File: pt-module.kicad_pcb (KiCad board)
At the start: 2 copper layers, 107 parts, among them J1 M12 in, J10 M12, J2 Ethercon out, J3 PWR in, J4 M12 out, J5 Ethercon out, J6 M12, J7 M12, J8 USB_OTG, J9 M12, SW1 pwr-source switch, SW10 SW_Push, SW11 SW_Push, SW12 SW_Push, SW13 SW_Push, SW2 SW_Push, SW3 SW_Push, SW4 SW_Push, SW5 SW_Push, SW6 SW_Push, SW7 SW_Push, SW8 SW_Push, SW9 SW_Push, U1 MCP16331, U10 LH1526, U2 MCP16331, U3 SN65HVD72, U4 SN65HVD72, U5 DG411, U6 LH1526, U7 FT230XS, U8 STM32F334R8Tx, U9 DG411

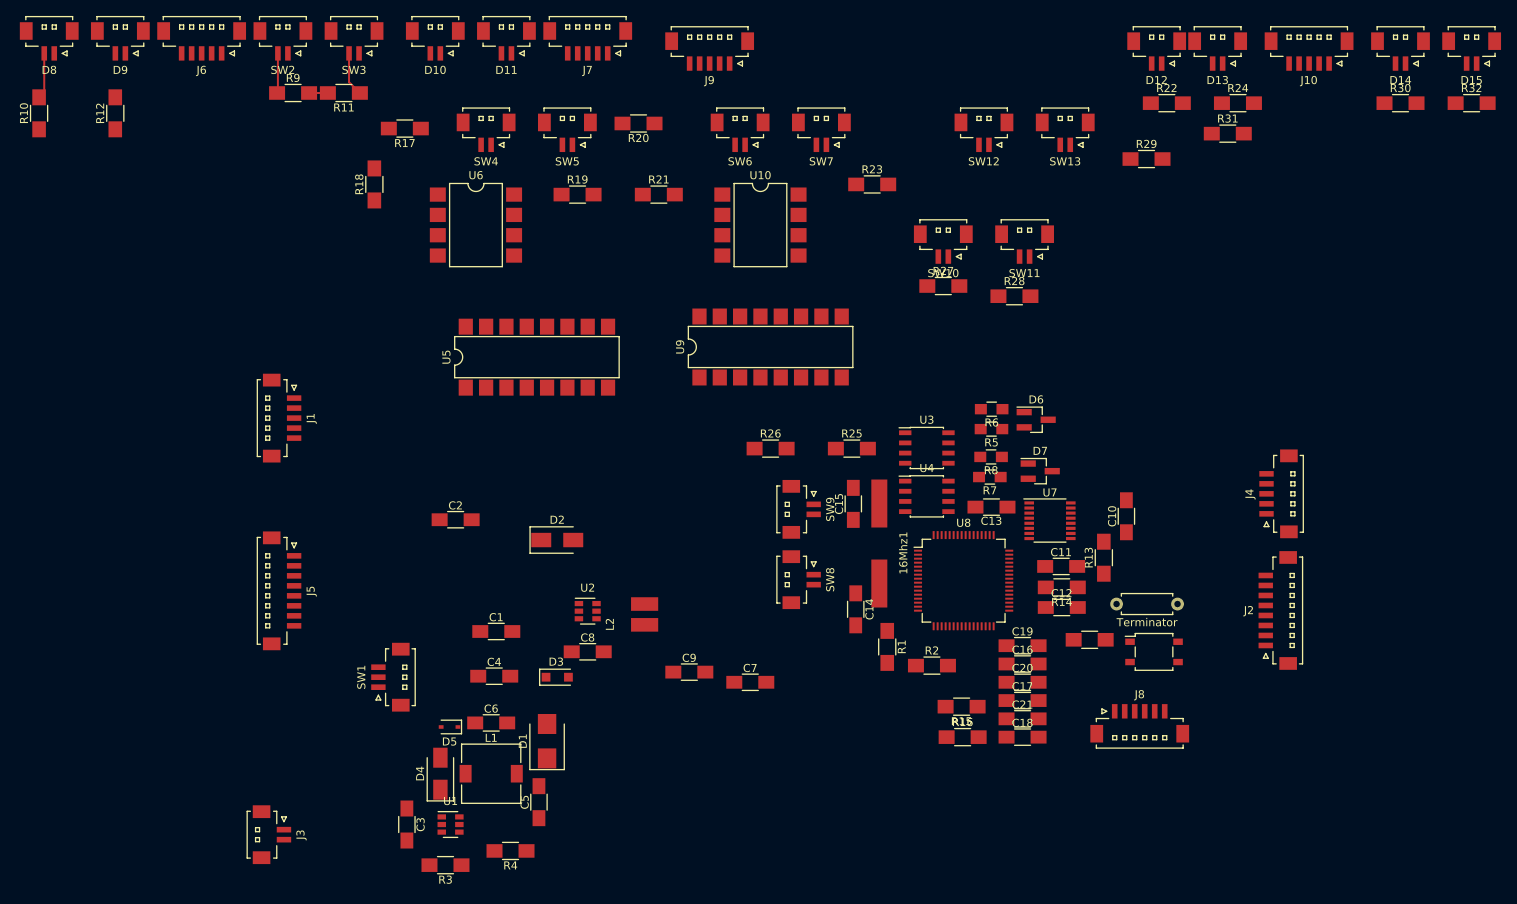
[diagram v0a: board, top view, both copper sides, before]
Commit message: Updated PCB
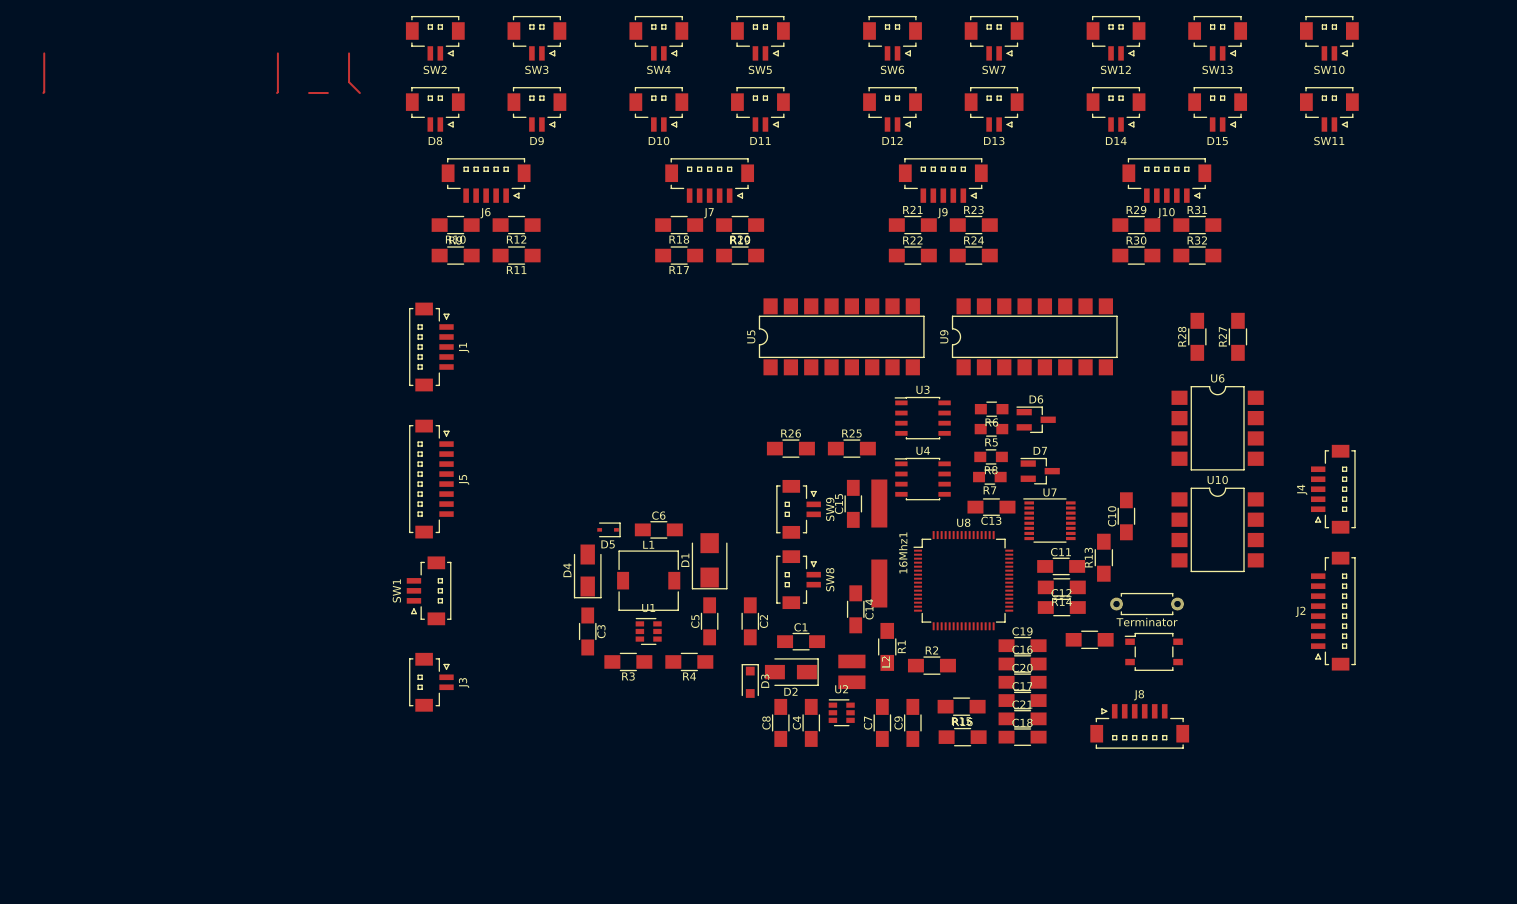
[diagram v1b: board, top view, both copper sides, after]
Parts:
- moved U6 96.1 mm to (180.3, 66.0)
- moved U10 68.7 mm to (180.3, 78.7)
- moved SW10 54.5 mm to (194.3, 17.8)
- moved R10 53.9 mm to (85.1, 40.6), turned to 180 degrees
- moved D9 52.8 mm to (95.2, 26.7)
- moved R12 52.1 mm to (92.7, 40.6), turned to 180 degrees
- moved D8 49.1 mm to (82.5, 26.7)
- moved SW11 41.5 mm to (194.3, 26.7)
- moved C4 40.1 mm to (129.5, 102.9), turned to 90 degrees
- moved J6 39.8 mm to (88.9, 35.6)
- moved R32 39.2 mm to (177.8, 44.5)
- moved C2 39.0 mm to (121.9, 90.2), turned to 270 degrees
- moved R18 38.4 mm to (113.0, 40.6), turned to 180 degrees
- moved U5 38.2 mm to (133.3, 54.6)
- moved C1 38.1 mm to (128.3, 92.7)
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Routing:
- net (no net): track 0.00 -> 17.8 mm
- net /PT module interface/prb1_rs_btn: track 5.51 -> 0.00 mm
- net Net-(D8-Pad2): track 4.99 -> 0.00 mm
- net /PT module interface/prb1_pwr_btn: track 4.99 -> 0.00 mm
- net +3V3: track 2.35 -> 0.00 mm
